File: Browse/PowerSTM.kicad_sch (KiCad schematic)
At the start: 3 parts, among them IC2 TCAN3414DRBR

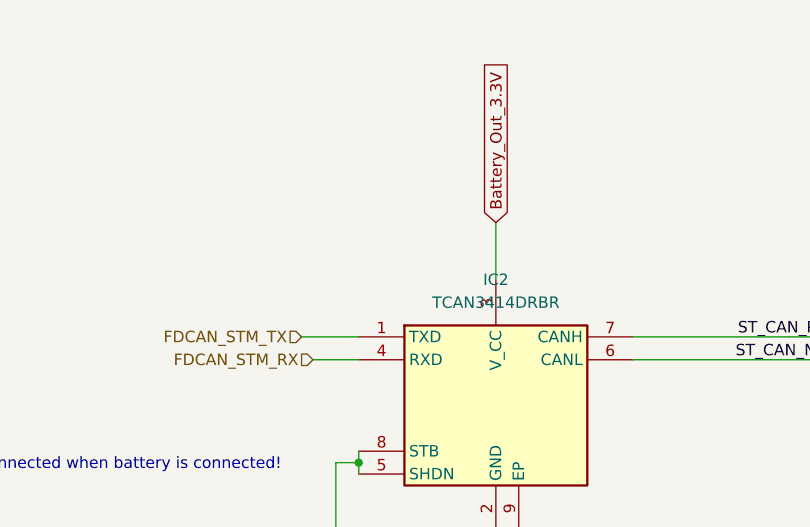
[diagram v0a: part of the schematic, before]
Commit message: Deploying to gh-pages from @ Nautilus-UUV/nautilus-mainboard-PCB@a81f7ffbfc5f9b51f47d7f388c30fcea2673b9ea 🚀
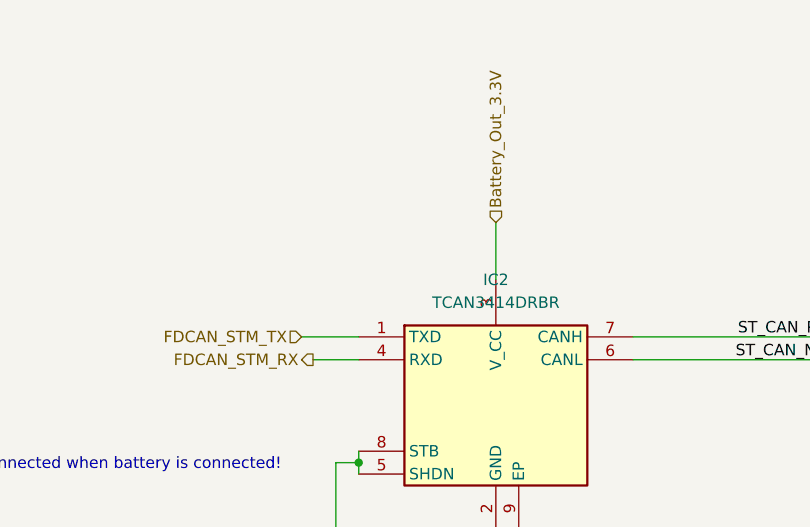
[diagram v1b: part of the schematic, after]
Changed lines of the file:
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@@
     (effects (font (size 1.27 1.27)) (justify right bottom))
-  )
-  (global_label "Battery_Out_3.3V" (shape input) (at 142.24 64.77 90) (fields_autoplaced)
-    (effects (font (size 1.27 1.27)) (justify left))
-    (property "Intersheetrefs" "${INTERSHEET_REFS}" (at 142.24 45.8192 90)
-      (effects (font (size 1.27 1.27)) (justify left) (hide yes))
-    )
   )
   (global_label "ST_CAN_N" (shape input) (at 226.06 86.36 0) (fields_autoplaced)
@@
     )
   )
-  (hierarchical_label "FDCAN_STM_RX" (shape input) (at 121.92 80.01 180)
+  (hierarchical_label "FDCAN_STM_RX" (shape output) (at 121.92 80.01 180)
     (effects (font (size 1.27 1.27)) (justify right))
   )
+  (hierarchical_label "Battery_Out_3.3V" (shape input) (at 142.24 64.77 90)
+    (effects (font (size 1.27 1.27)) (justify left))
+  )
   (hierarchical_label "FDCAN_STM_TX" (shape input) (at 120.65 77.47 180)
